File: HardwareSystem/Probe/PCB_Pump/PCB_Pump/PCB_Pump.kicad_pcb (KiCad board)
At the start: 2 copper layers, 20.8 x 66.8 mm, 4 parts, among them Q1 IRF510

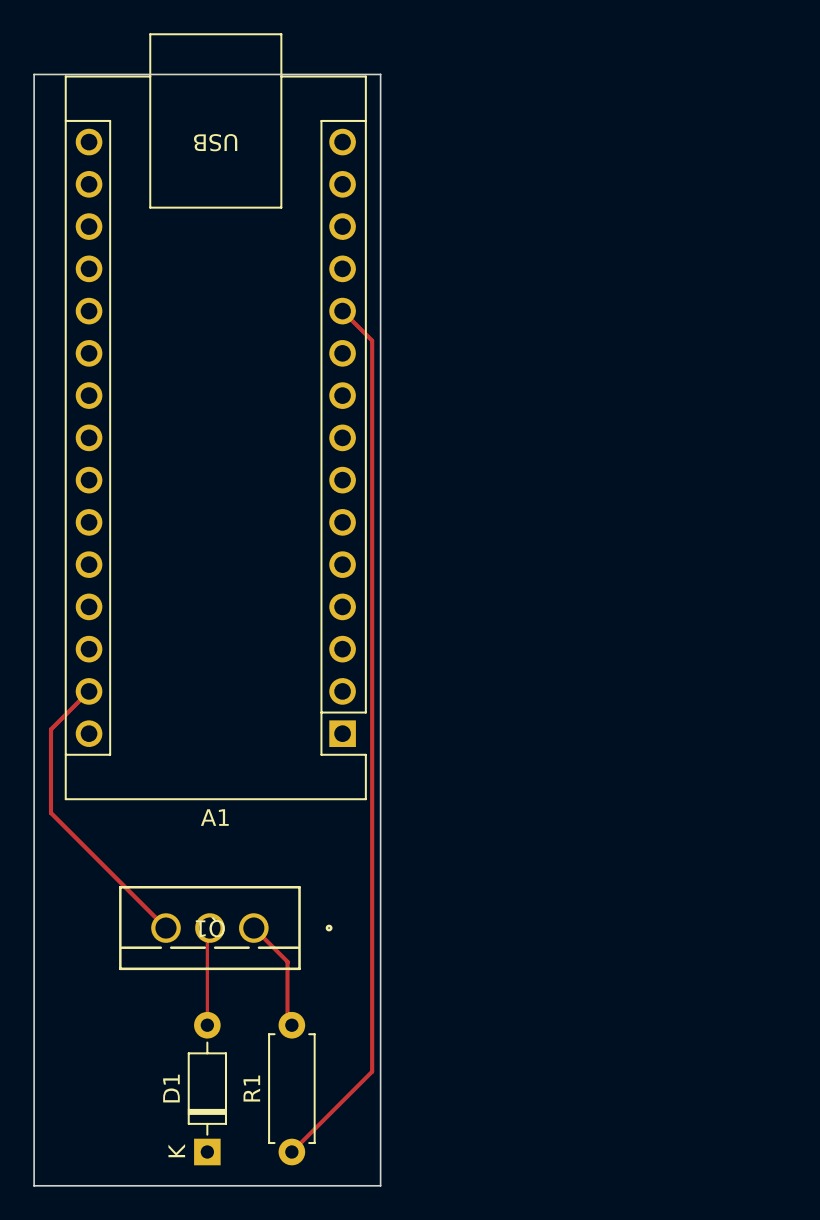
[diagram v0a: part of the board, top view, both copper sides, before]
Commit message: pump pcb work
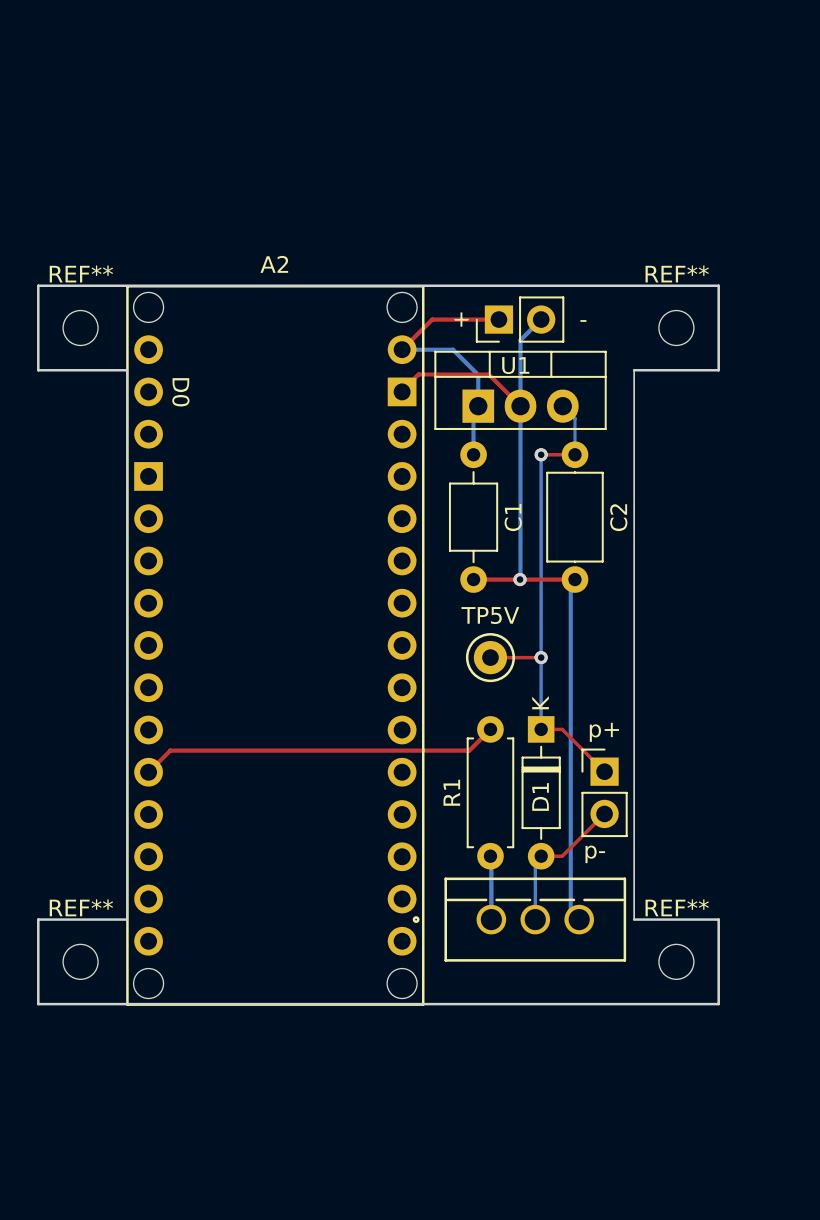
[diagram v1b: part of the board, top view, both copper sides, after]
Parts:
- removed A1: Arduino_Nano_Every, Module:Arduino_Nano
- added +: PinHeader_1x02_P2.54mm_Vertical, Connector_PinHeader_2.54mm:PinHeader_1x02_P2.54mm_Vertical, F.Cu at (169.2, 42.9)
- added A2: Arduino_Nano_ESP32_Socket, footprints:Arduino_Nano_ESP32_Socket, F.Cu at (155.7, 84.1)
- added C1: 0.1 uF, Capacitor_THT:C_Axial_L3.8mm_D2.6mm_P7.50mm_Horizontal, F.Cu at (167.6, 51.1)
- added C2: 10 uF, Capacitor_THT:C_Axial_L5.1mm_D3.1mm_P7.50mm_Horizontal, F.Cu at (173.7, 51.1)
- added REF**: MountingHole_2.1mm, MountingHole:MountingHole_2.1mm, F.Cu at (179.8, 43.4)
- added REF**: MountingHole_2.1mm, MountingHole:MountingHole_2.1mm, F.Cu at (144.0, 43.4)
- added REF**: MountingHole_2.1mm, MountingHole:MountingHole_2.1mm, F.Cu at (179.8, 81.5)
- added REF**: MountingHole_2.1mm, MountingHole:MountingHole_2.1mm, F.Cu at (144.0, 81.5)
- added TP5V: TestPoint_Keystone_5000-5004_Miniature, TestPoint:TestPoint_Keystone_5000-5004_Miniature, F.Cu at (168.7, 63.2)
- added U1: LM2937xT, Package_TO_SOT_THT:TO-220-3_Vertical, F.Cu at (167.9, 48.1)
- added p+: PinHeader_1x02_P2.54mm_Vertical, Connector_PinHeader_2.54mm:PinHeader_1x02_P2.54mm_Vertical, F.Cu at (175.5, 70.1)
- moved D1 32.4 mm to (171.7, 67.6), turned to -90 degrees
- moved R1 28.1 mm to (168.7, 67.6), turned to -90 degrees
- moved Q1 14.3 mm to (168.7, 79.0), turned to 0 degrees
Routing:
- net GND: track 18.0 -> 51.4 mm, vias 0 -> 1
- net Net-(A2-PadD8): track 53.3 -> 21.6 mm
- net pump+: track 0.00 -> 29.7 mm, vias 0 -> 2
- net 9V: track 0.00 -> 16.7 mm
- net Net-(Q1-G): track 6.79 -> 3.83 mm
- net pump-: track 5.91 -> 8.82 mm
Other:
- board size 20.8 x 66.8 mm -> 40.9 x 43.2 mm
- board text added: "-"
- board text added: "p-"
